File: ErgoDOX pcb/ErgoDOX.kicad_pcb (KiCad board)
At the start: 2 copper layers, 182.8 x 158.9 mm, 77 parts, among them J1 USB, J2 3.5mm, J3 JMP, J4 JMP, SW0:10 SW0:3, SW0:11 SW0:2, SW0:12 SW0:1, SW0:7 SW0:6, SW0:8 SW0:5, SW0:9 SW0:4, SW1:10 SW1:3, SW1:11 SW1:2, SW1:12 SW1:1, SW1:13 SW1:0, SW1:9 SW1:4, SW2:10 SW2:3, SW2:11 SW2:2, SW2:12 SW2:1, SW2:13 SW2:0, SW2:7 SW2:6, SW2:8 SW2:5, SW2:9 SW2:4, SW3:10 SW3:3, SW3:11 SW3:2, SW3:12 SW3:1, SW3:13 SW3:0, SW3:8 SW3:5, SW3:9 SW3:4, SW4:10 SW4:3, SW4:11 SW4:2, SW4:12 SW4:1, SW4:13 SW4:0, SW4:7 SW4:6, SW4:8 SW4:5, SW4:9 SW4:4, SW5:10 SW5:3, SW5:11 SW5:2, SW5:12 SW5:1, SW5:13 SW5:0, SW5:7 SW5:6, SW5:8 SW5:5, SW5:9 SW5:4, U1 TEENSY2.0, U2 MCP23018

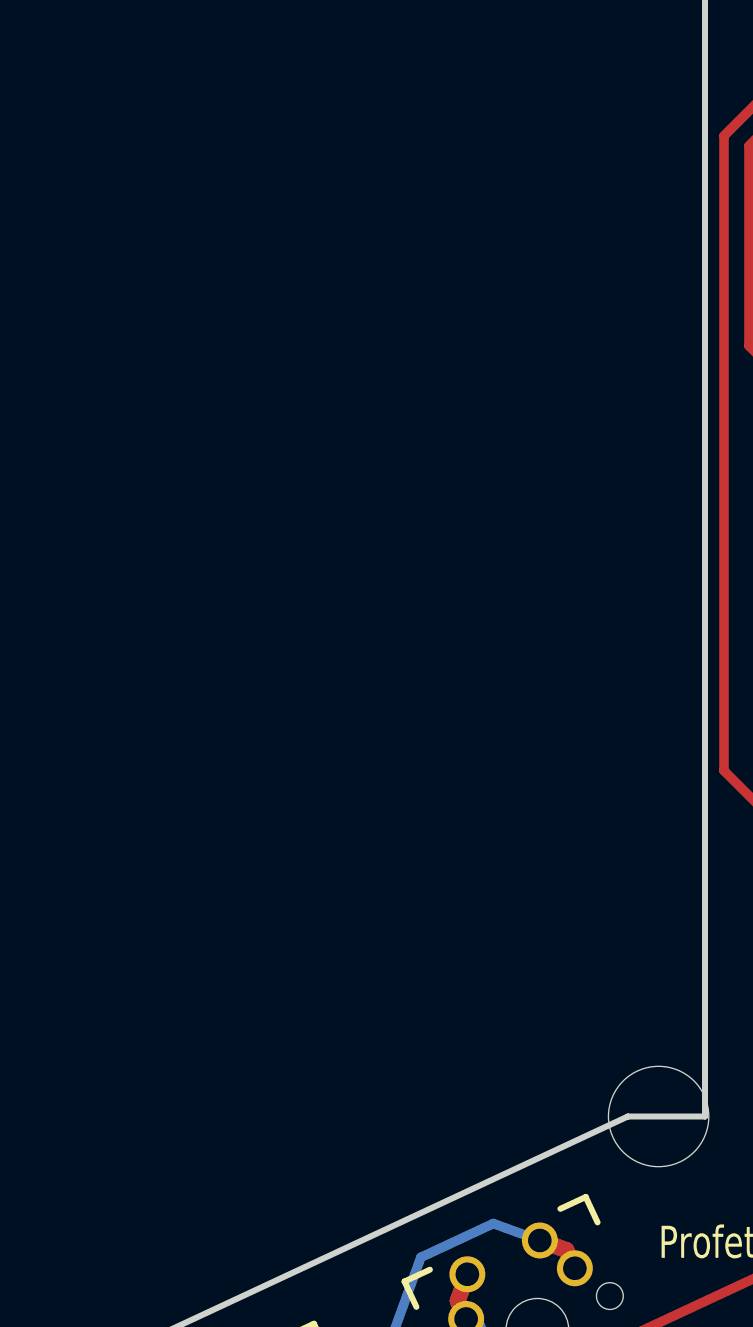
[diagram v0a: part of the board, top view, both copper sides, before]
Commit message: adding cringe
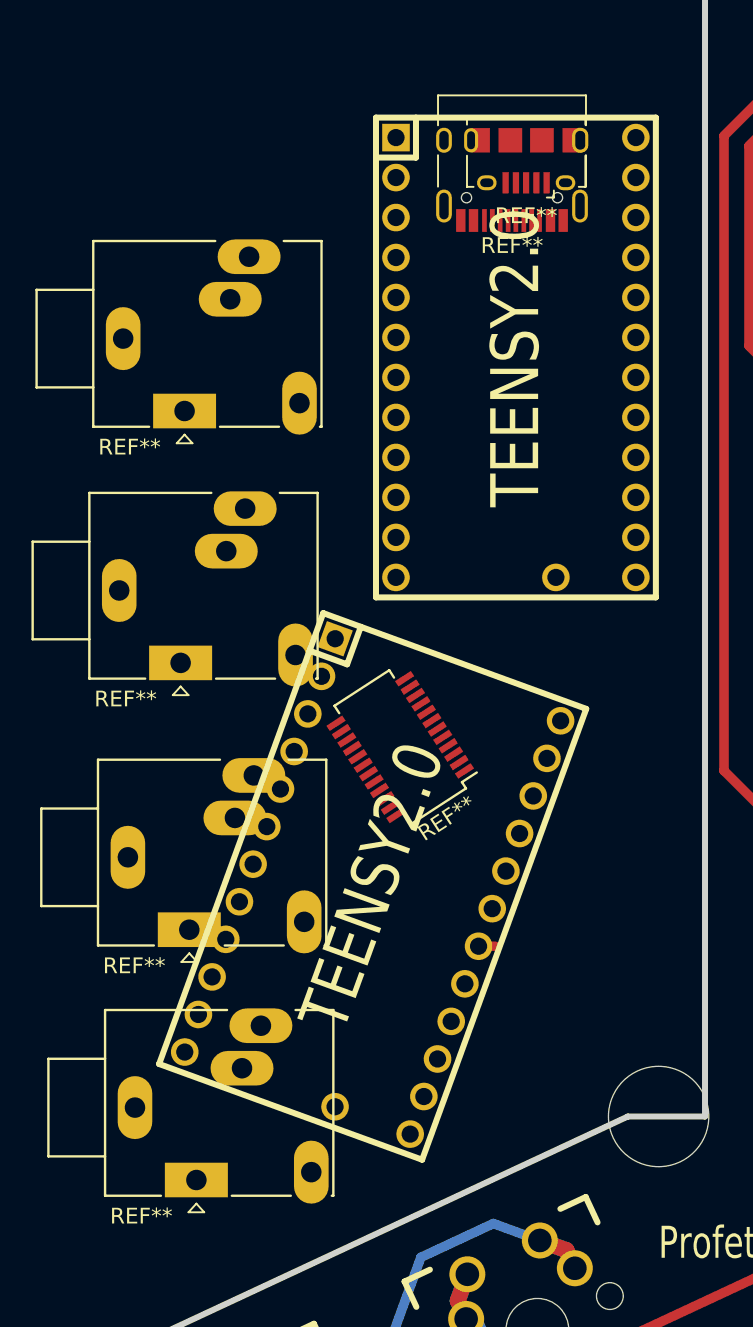
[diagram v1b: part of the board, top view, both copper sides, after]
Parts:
- added REF**: Jack_3.5mm_Ledino_KB3SPRS_Horizontal, Connector_Audio:Jack_3.5mm_Ledino_KB3SPRS_Horizontal, F.Cu at (29.6, 76.8)
- added REF**: Jack_3.5mm_Ledino_KB3SPRS_Horizontal, Connector_Audio:Jack_3.5mm_Ledino_KB3SPRS_Horizontal, F.Cu at (29.3, 92.8)
- added REF**: Jack_3.5mm_Ledino_KB3SPRS_Horizontal, Connector_Audio:Jack_3.5mm_Ledino_KB3SPRS_Horizontal, F.Cu at (29.9, 109.8)
- added REF**: Jack_3.5mm_Ledino_KB3SPRS_Horizontal, Connector_Audio:Jack_3.5mm_Ledino_KB3SPRS_Horizontal, F.Cu at (30.3, 125.7)
- added REF**: USB_Micro-B_Amphenol_10118194_Horizontal, Connector_USB:USB_Micro-B_Amphenol_10118194_Horizontal, F.Cu at (51.2, 61.0)
- added REF**: USB_C_Receptacle_HRO_TYPE-C-31-M-12, Connector_USB:USB_C_Receptacle_HRO_TYPE-C-31-M-12, F.Cu at (50.4, 60.7)
- added REF**: SSOP-24_3.9x8.7mm_P0.635mm, Package_SO:SSOP-24_3.9x8.7mm_P0.635mm, F.Cu at (43.2, 98.2)
- added U1: TEENSY2.0, ErgoDOX pcb:TEENSY_2.0_WITH_RESET, F.Cu at (41.5, 107.0)
- added U1: TEENSY2.0, ErgoDOX pcb:TEENSY_2.0_WITH_RESET, F.Cu at (50.6, 73.5)
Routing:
- net (no net): track 0.00 -> 1.07 mm
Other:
- board text added: "ErgoCringe 2021 (name subject to be changed)"
